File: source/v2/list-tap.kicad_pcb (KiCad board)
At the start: 2 copper layers, 37.4 x 55.5 mm, 59 parts, among them J1 TYPE-C-31-M-12, SW1 SKRKAEE020, SW2 SKRKAEE020, SW3 PTS815 SJM 250 SMTR LFS, U1 DM-OLED096-636, U3 USBLC6-2SC6Y, U4 TPS2116DRLR, U5 TPS63805YFFR, U6 ESP32-C3-WROOM-02-N4

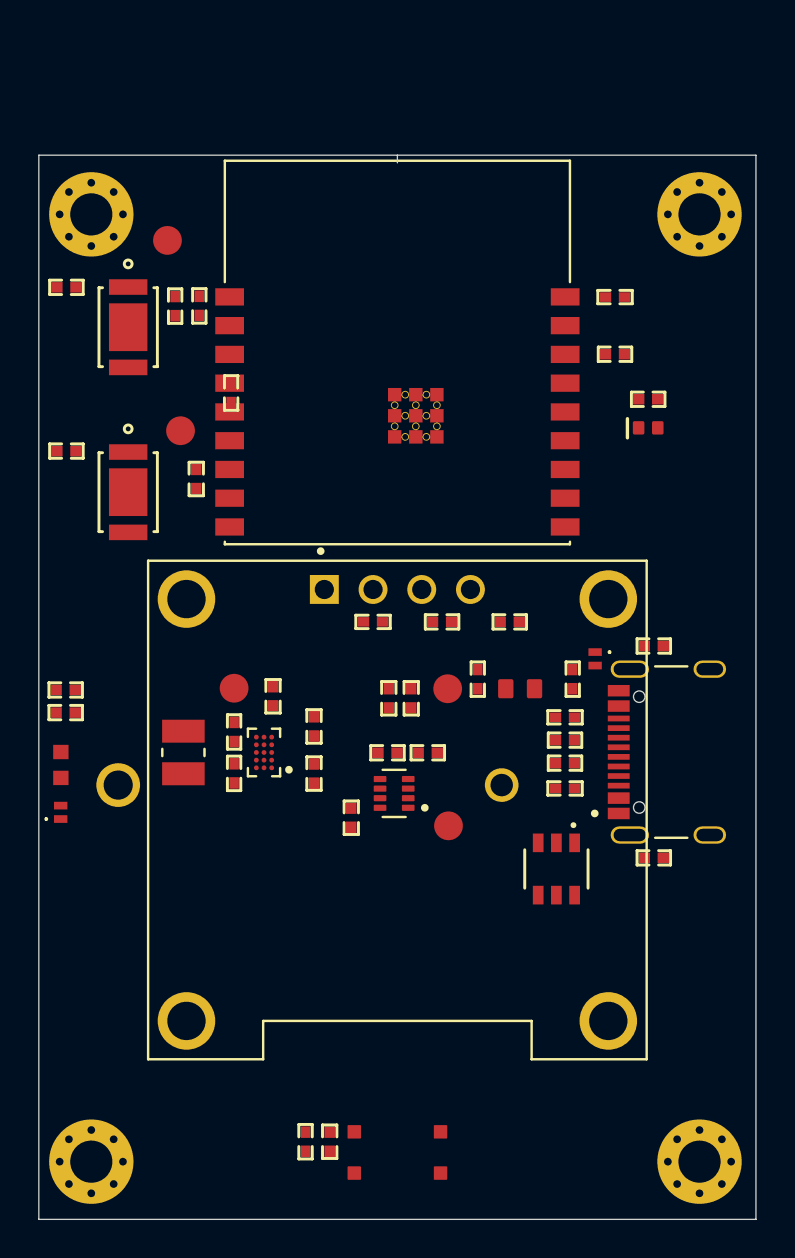
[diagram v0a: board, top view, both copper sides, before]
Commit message: layout r3
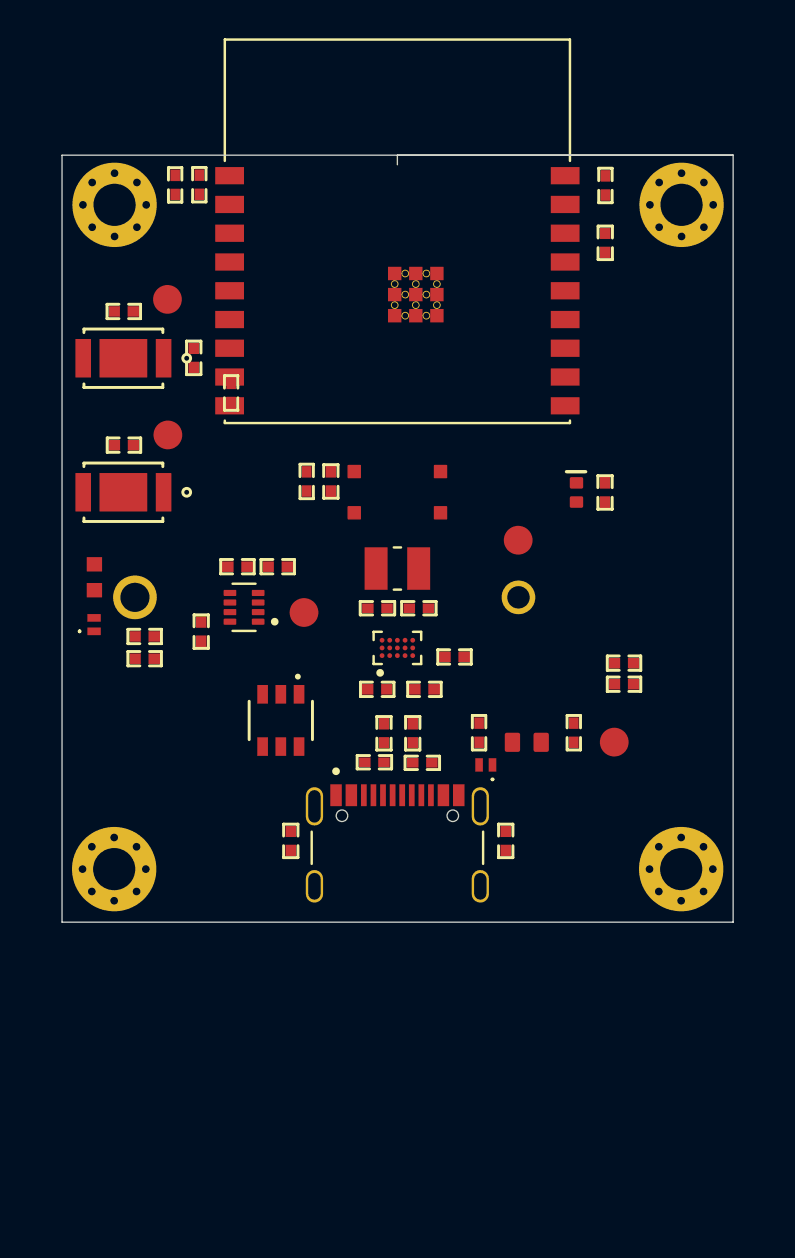
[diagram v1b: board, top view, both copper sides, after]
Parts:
- removed C12: 100n 50V, list-tap:CAPC1005X04L
- removed R25, R26: 4k7, list-tap:RESC1005X04L
- removed U1: DM-OLED096-636, list-tap:MODULE_DM-OLED096-636
- moved C16 34.4 mm to (147.5, 73.9)
- moved R23 34.4 mm to (148.8, 73.9)
- moved SW3 34.4 mm to (152.2, 74.5)
- moved R1 19.0 mm to (146.7, 92.7), turned to 90 degrees
- moved J1 17.7 mm to (152.2, 95.1), turned to 0 degrees
- moved TP3 16.7 mm to (158.5, 77.0), turned to 0 degrees
- moved U3 16.3 mm to (146.2, 86.4)
- moved H4 15.3 mm to (137.5, 94.2)
- moved H3 15.3 mm to (167.0, 94.2)
- moved L1 14.7 mm to (152.2, 78.5), turned to 180 degrees
- moved TP4 13.4 mm to (147.4, 80.8)
- moved R2 12.8 mm to (157.9, 92.7), turned to 90 degrees
- moved R28 12.5 mm to (142.0, 81.8)
- moved R29 12.5 mm to (143.9, 78.4)
- moved U4 12.5 mm to (144.2, 80.5)
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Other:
- board size 37.4 x 55.5 mm -> 35 x 40 mm
